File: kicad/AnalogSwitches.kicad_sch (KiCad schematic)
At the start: 63 parts

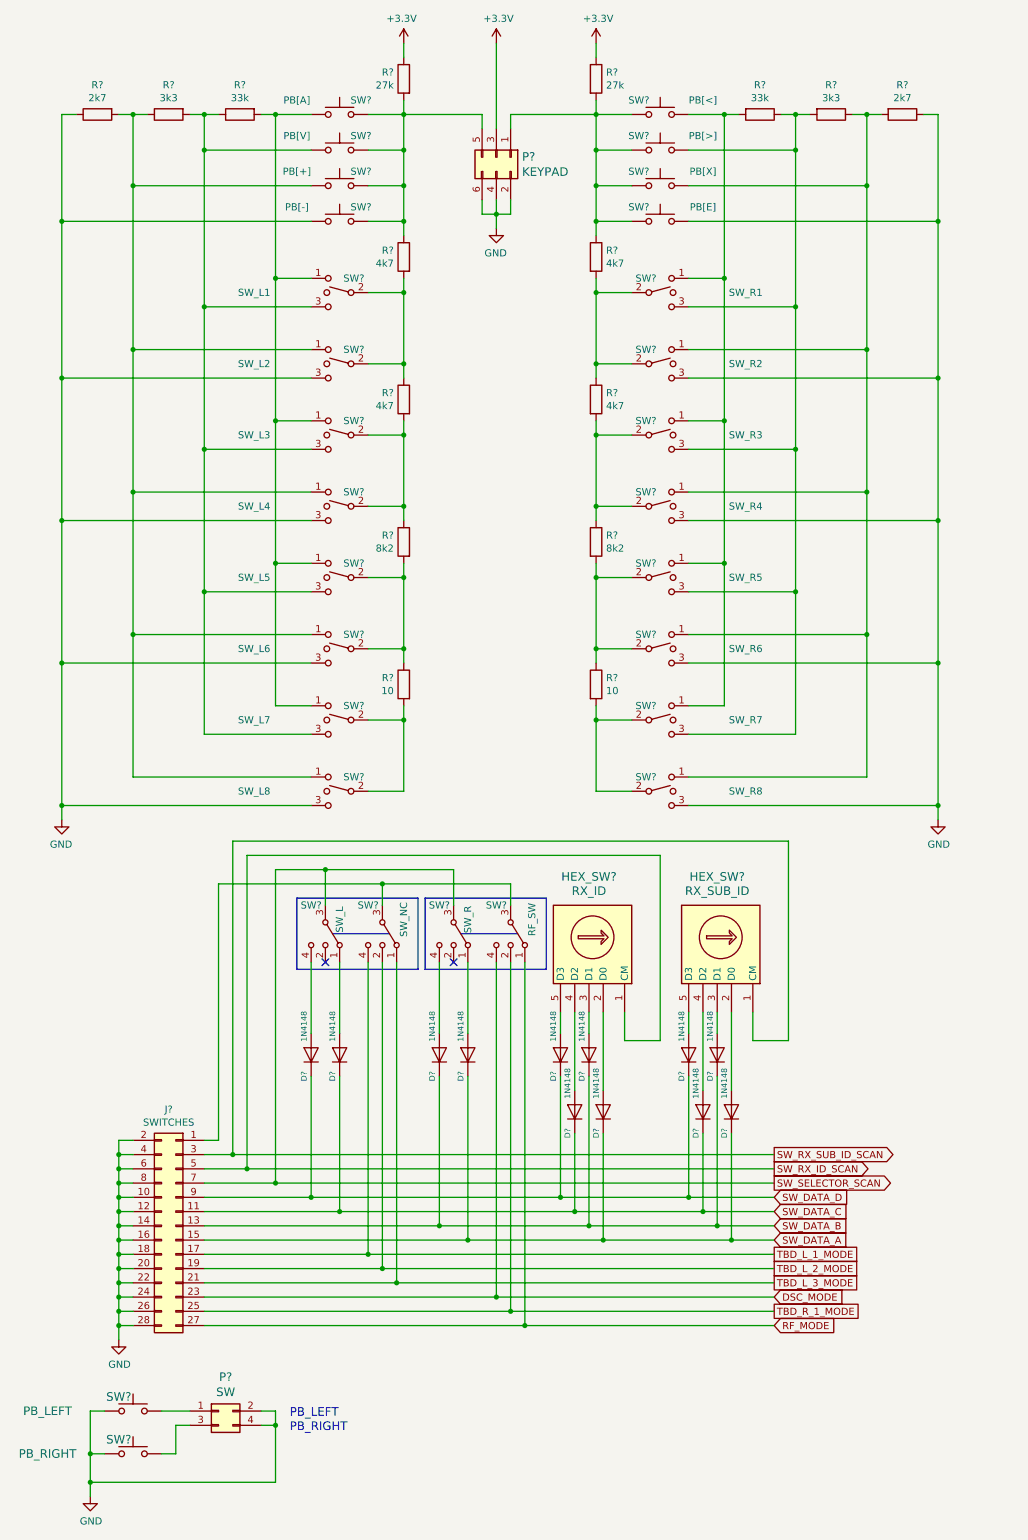
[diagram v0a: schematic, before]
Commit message: Optimizing power lines
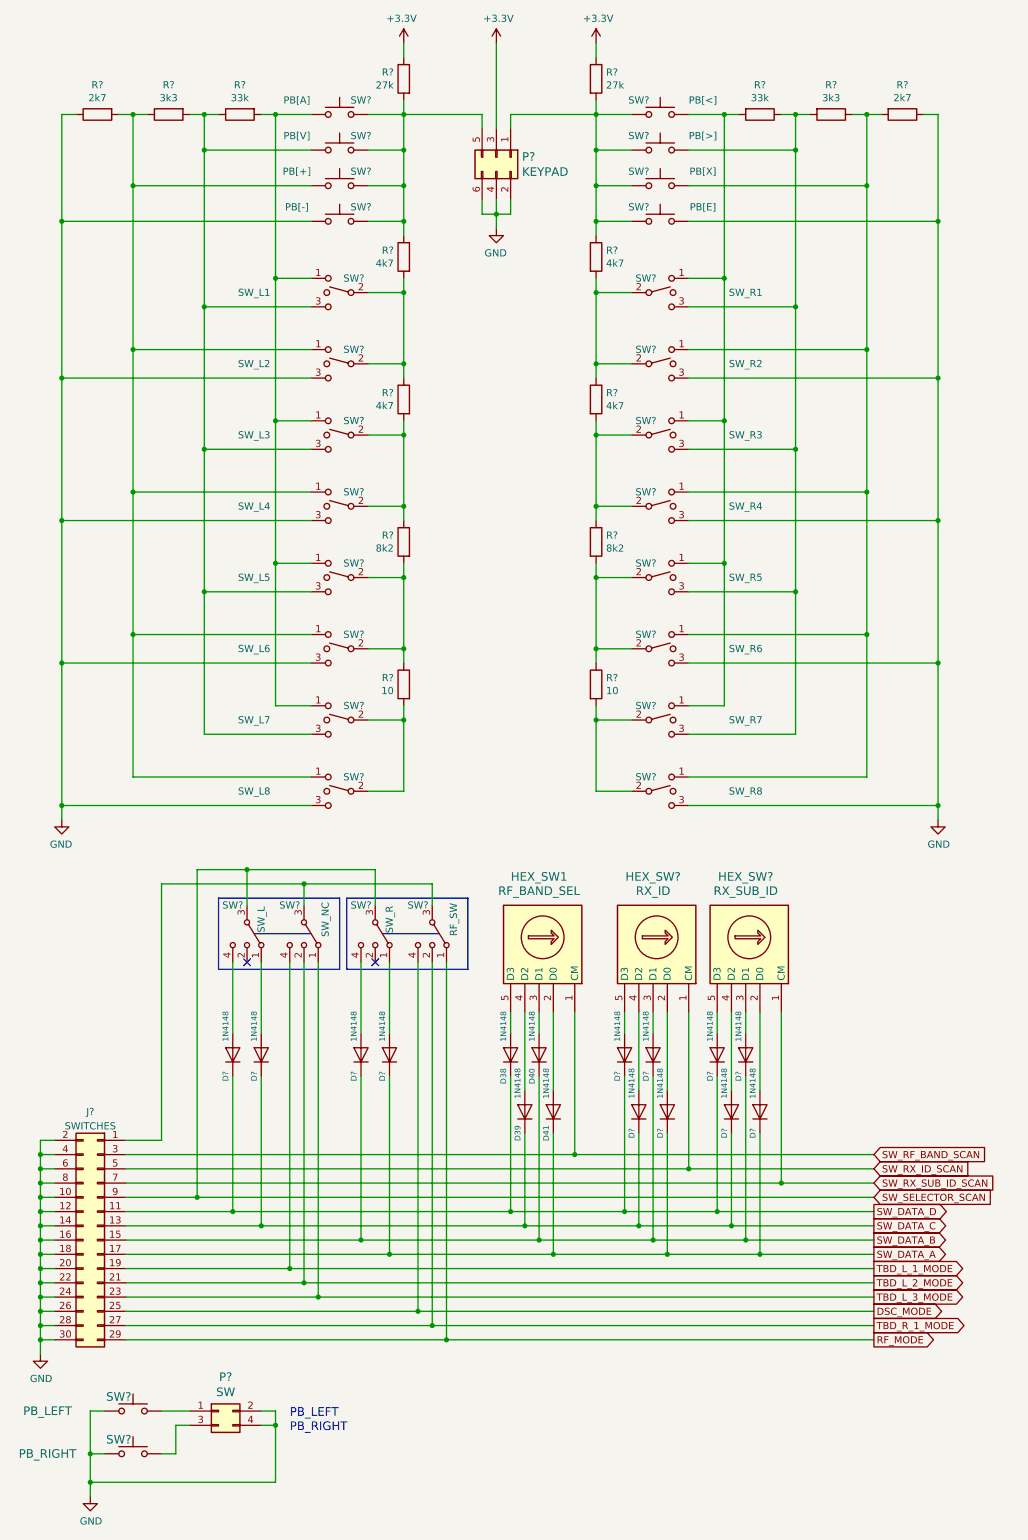
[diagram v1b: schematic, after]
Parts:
- removed J?: SWITCHES, symbol conn:Conn_02x14_Odd_Even
- added D38, D39, D40, D41: 1N4148, Diodes_THT:D_5W_P5.08mm_Vertical_KathodeUp, symbol RCTX-rescue:D-device
- added HEX_SW1: RF_BAND_SEL, Buttons_Switches_THT:Nidec_Copal_SH-7010C, symbol RCTX-rescue:SW_Coded-switches
- added J?: SWITCHES, symbol Connector_Generic:Conn_02x15_Odd_Even
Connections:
- net DSC_MODE: now also J?.25 (Pin_25)
- net GND: now also J?.10 (Pin_10), J?.12 (Pin_12), J?.14 (Pin_14), J?.16 (Pin_16), J?.18 (Pin_18), J?.2 (Pin_2), J?.20 (Pin_20), J?.22 (Pin_22), J?.24 (Pin_24), J?.26 (Pin_26), J?.28 (Pin_28), J?.30 (Pin_30), J?.4 (Pin_4), J?.6 (Pin_6), J?.8 (Pin_8)
- net RF_MODE: now also J?.29 (Pin_29)
- net SW_DATA_A: now also D41.1 (K), J?.17 (Pin_17)
- net SW_DATA_B: now also D40.1 (K), J?.15 (Pin_15)
- net SW_DATA_C: now also D39.1 (K), J?.13 (Pin_13)
- net SW_DATA_D: now also D38.1 (K), J?.11 (Pin_11)
- net SW_RX_ID_SCAN: now also J?.5 (Pin_5)
- net SW_RX_SUB_ID_SCAN: now also J?.7 (Pin_7)
- net SW_SELECTOR_SCAN: now also J?.9 (Pin_9)
- net TBD_L_1_MODE: now also J?.19 (Pin_19)
- net TBD_L_2_MODE: now also J?.21 (Pin_21)
- net TBD_L_3_MODE: now also J?.23 (Pin_23)
- net TBD_R_1_MODE: now also J?.27 (Pin_27)
- net at SW?.3, SW?.3: now also J?.1 (Pin_1)
- new net: D41.2 (A), HEX_SW1.2 (D0)
- new net: D38.2 (A), HEX_SW1.5 (D3)
- new net: D39.2 (A), HEX_SW1.4 (D2)
- new net: D40.2 (A), HEX_SW1.3 (D1)
- new net SW_RF_BAND_SCAN: HEX_SW1.1 (CM), J?.3 (Pin_3)
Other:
- moved on the sheet: D?, HEX_SW?, SW?
